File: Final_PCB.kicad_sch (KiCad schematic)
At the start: 31 parts, among them J1 USB_C_Receptacle_USB2.0_16P, J2 Conn_ARM_SWD_TagConnect_TC2030, J3 DE15_Pins_HighDensity_Mountin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, SW1 SW_Push, U1 RP2040, U2 USBLC6-2SC6, U3 SPX3819M5-L-3-3, Y1 12MHz

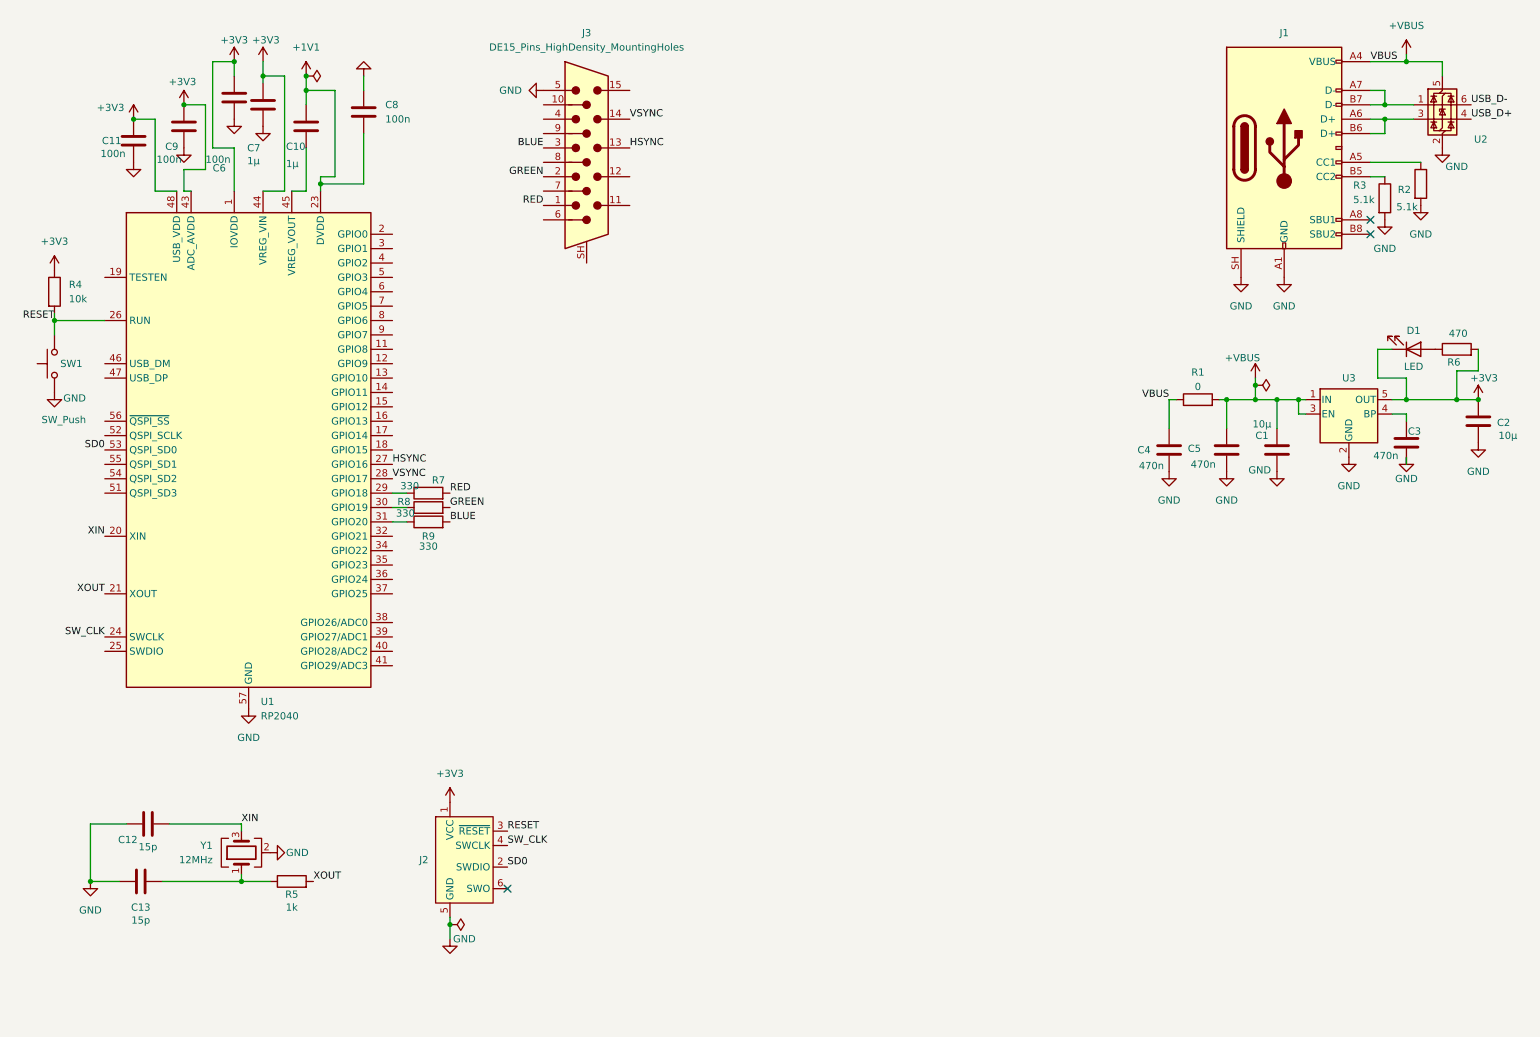
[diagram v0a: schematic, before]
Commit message: Routing almost done
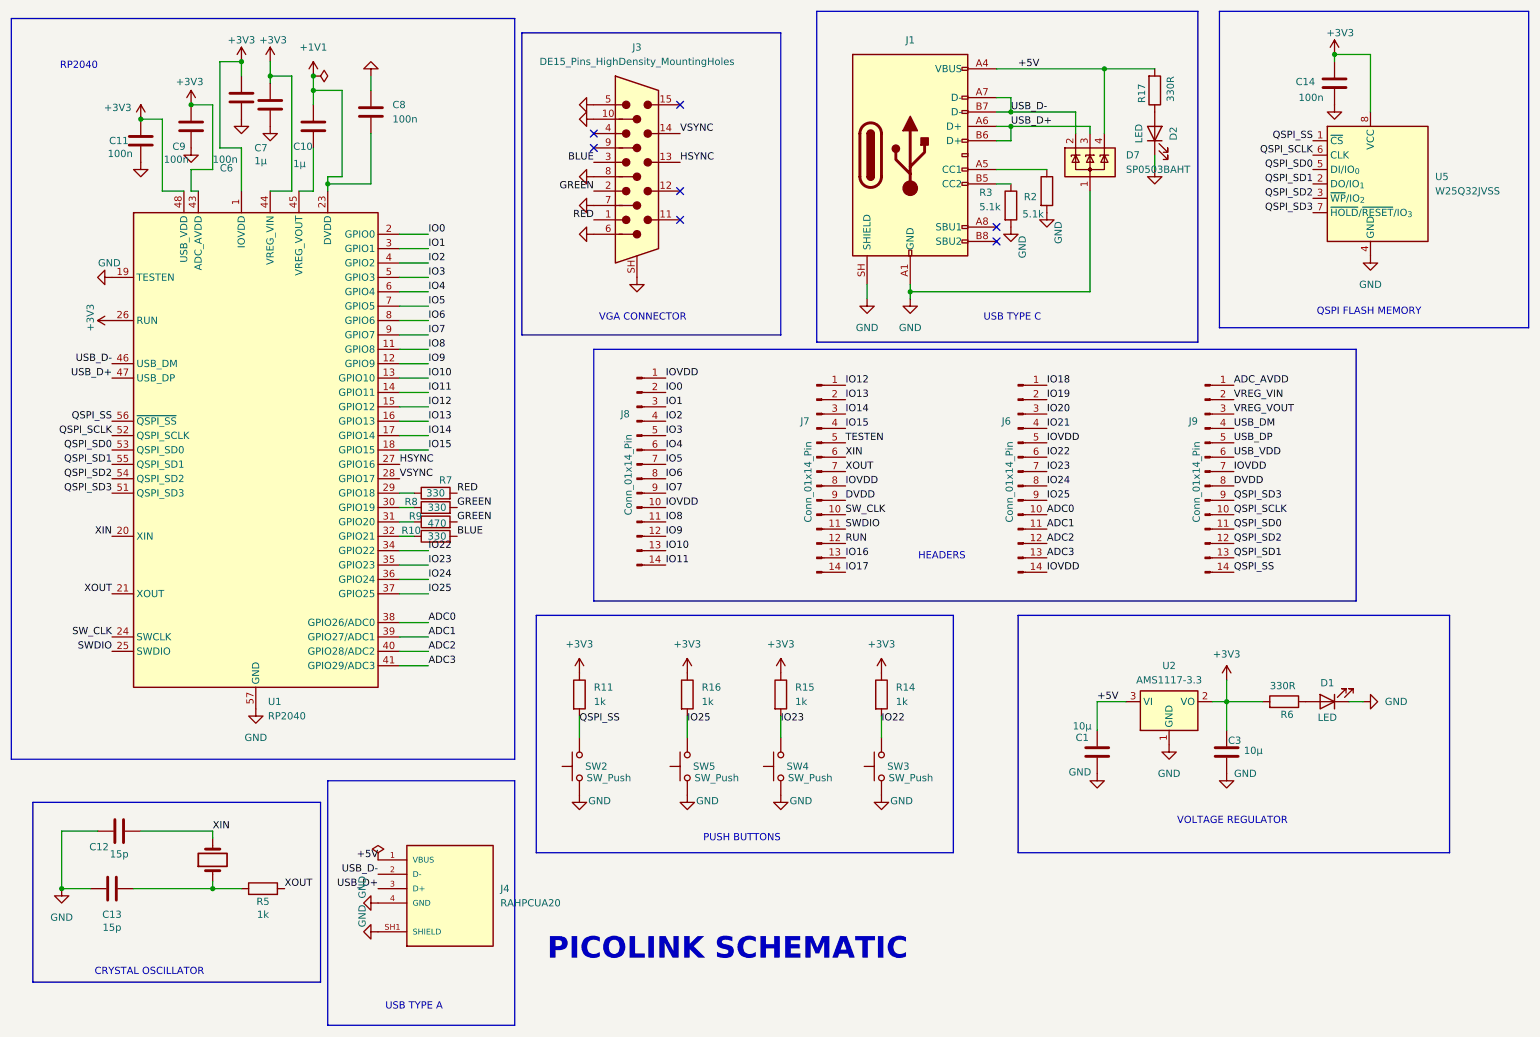
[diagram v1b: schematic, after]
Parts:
- removed C2: 10µ, Capacitor_SMD:C_0603_1608Metric, symbol Device:C
- removed C4, C5: 470n, Capacitor_SMD:C_0603_1608Metric, symbol Device:C
- removed J2: Conn_ARM_SWD_TagConnect_TC2030, Connector:Tag-Connect_TC2030-IDC-FP_2x03_P1.27mm_Vertical, symbol Connector:Conn_ARM_SWD_TagConnect_TC2030
- removed R1: 0, Resistor_SMD:R_0603_1608Metric, symbol Device:R
- removed R4: 10k, Resistor_SMD:R_0603_1608Metric, symbol Device:R
- removed SW1: SW_Push, Button_Switch_SMD:SW_SPST_B3U-1000P, symbol Switch:SW_Push
- removed U2: USBLC6-2SC6, Package_TO_SOT_SMD:SOT-23-6, symbol Power_Protection:USBLC6-2SC6
- removed U3: SPX3819M5-L-3-3, Package_TO_SOT_SMD:SOT-23-5, symbol Regulator_Linear:SPX3819M5-L-3-3
- removed Y1: 12MHz, Crystal:Crystal_SMD_5032-4Pin_5.0x3.2mm, symbol Device:Crystal_GND24
- added C14: 100n, Capacitor_SMD:C_0805_2012Metric, symbol Device:C
- added D2: LED, LED_SMD:LED_0805_2012Metric, symbol Device:LED
- added D7: SP0503BAHT, Package_TO_SOT_SMD:SOT-143, symbol Power_Protection:SP0503BAHT
- added J4: RAHPCUA20, RAHPCUA20:SWITCHCRAFT_RAHPCUA20, symbol RAHPCUA20:RAHPCUA20
- added J6, J7, J8, J9: Conn_01x14_Pin, Connector_PinHeader_1.27mm:PinHeader_1x14_P1.27mm_Vertical, symbol Connector:Conn_01x14_Pin
- added R10: 330, Resistor_SMD:R_0805_2012Metric, symbol Device:R
- added R11, R14, R15, R16: 1k, Resistor_SMD:R_0805_2012Metric, symbol Device:R
- added R17: 330R, Resistor_SMD:R_0805_2012Metric, symbol Device:R
- added SW2, SW3, SW4, SW5: SW_Push, Button_Switch_SMD:SW_SPST_B3U-1000P, symbol Switch:SW_Push
- added U2: AMS1117-3.3, Package_TO_SOT_SMD:SOT-223-3_TabPin2, symbol Regulator_Linear:AMS1117-3.3
- added U5: W25Q32JVSS, Package_SO:SOIC-8_5.3x5.3mm_P1.27mm, symbol Memory_Flash:W25Q32JVSS
- added Y2: Crystal, Crystal:Crystal_SMD_5032-2Pin_5.0x3.2mm, symbol Device:Crystal
- C1, C10, C11, C12, C13, C6, C7, C8, C9: footprint Capacitor_SMD:C_0603_1608Metric -> Capacitor_SMD:C_0805_2012Metric
- C3: value 470n -> 10µ; footprint Capacitor_SMD:C_0603_1608Metric -> Capacitor_SMD:C_0805_2012Metric
- J1: footprint Connector_USB:USB_C_Receptacle_G-Switch_GT-USB-7010ASV -> Connector_USB:USB_C_Receptacle_GCT_USB4105-xx-A_16P_TopMnt_Horizontal
- J3: footprint (none) -> Connector_Dsub:DSUB-15-HD_Socket_Horizontal_P2.29x1.90mm_EdgePinOffset3.03mm_Housed_MountingHolesOffset4.94mm
- R2, R3, R5: footprint Resistor_SMD:R_0603_1608Metric -> Resistor_SMD:R_0805_2012Metric
- R6: value 470 -> 330R; footprint Resistor_SMD:R_0603_1608Metric -> Resistor_SMD:R_0805_2012Metric
- R7, R8: footprint (none) -> Resistor_SMD:R_0805_2012Metric
- R9: value 330 -> 470; footprint (none) -> Resistor_SMD:R_0805_2012Metric
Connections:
- net RESET is gone; now on net +3V3: U1.26 (RUN)
- net +3V3: now also C3.1, C14.1, R11.1, R14.1, R15.1, R16.1, U2.2 (VO), U5.8 (VCC); no longer D1.1 (K)
- net BLUE: now also R10.2; no longer R9.2
- net GND: now also D1.1 (K), J3.10, J3.6, J3.7, J3.8, J3.SH, U1.19 (TESTEN), C14.2, D2.1 (K), D7.1 (A), J4.4 (GND), J4.SH1 (SHIELD), J4.SH2 (SHIELD), SW2.1, SW3.1, SW4.1, SW5.1, U2.1 (GND), U5.4 (GND)
- net GREEN: now also R9.2
- net SW_CLK: now also J7.10 (Pin_10)
- net USB_D+: now also J1.A6 (D+), J1.B6 (D+), U1.47 (USB_DP), D7.3 (K), J4.3 (D+)
- net USB_D-: now also J1.A7 (D-), J1.B7 (D-), U1.46 (USB_DM), D7.2 (K), J4.2 (D-)
- net XIN: now also J7.6 (Pin_6), Y2.2
- net XOUT: now also J7.7 (Pin_7)
- net at C13.2, R5.1: now also Y2.1
- net IO8: now reaches U1.11 (GPIO8)
- net IO8: now also J8.11 (Pin_11)
- net IO9: now reaches U1.12 (GPIO9)
- net IO9: now also J8.12 (Pin_12)
- net IO10: now reaches U1.13 (GPIO10)
- net IO10: now also J8.13 (Pin_13)
- net IO11: now reaches U1.14 (GPIO11)
- net IO11: now also J8.14 (Pin_14)
- net IO12: now reaches U1.15 (GPIO12)
- net IO12: now also J7.1 (Pin_1)
- net IO13: now reaches U1.16 (GPIO13)
- net IO13: now also J7.2 (Pin_2)
- net IO14: now reaches U1.17 (GPIO14)
- net IO14: now also J7.3 (Pin_3)
- net IO15: now reaches U1.18 (GPIO15)
- net IO15: now also J7.4 (Pin_4)
- net IO0: now reaches U1.2 (GPIO0)
- net IO0: now also J8.2 (Pin_2)
- net SWDIO: now reaches U1.25 (SWDIO)
- net SWDIO: now also J7.11 (Pin_11)
- net IO1: now reaches U1.3 (GPIO1)
- net IO1: now also J8.3 (Pin_3)
- net at U1.32 (GPIO21): now also R10.1
- net IO22: now reaches U1.34 (GPIO22)
- net IO22: now also J6.6 (Pin_6), R14.2, SW3.2
- net IO23: now reaches U1.35 (GPIO23)
- net IO23: now also J6.7 (Pin_7), R15.2, SW4.2
- net IO24: now reaches U1.36 (GPIO24)
- net IO24: now also J6.8 (Pin_8)
- net IO25: now reaches U1.37 (GPIO25)
- net IO25: now also J6.9 (Pin_9), R16.2, SW5.2
- net ADC0: now reaches U1.38 (GPIO26/ADC0)
- net ADC0: now also J6.10 (Pin_10)
- net ADC1: now reaches U1.39 (GPIO27/ADC1)
- net ADC1: now also J6.11 (Pin_11)
- net IO2: now reaches U1.4 (GPIO2)
- net IO2: now also J8.4 (Pin_4)
- net ADC2: now reaches U1.40 (GPIO28/ADC2)
- net ADC2: now also J6.12 (Pin_12)
- net ADC3: now reaches U1.41 (GPIO29/ADC3)
- net ADC3: now also J6.13 (Pin_13)
- net IO3: now reaches U1.5 (GPIO3)
- net IO3: now also J8.5 (Pin_5)
- net QSPI_SD3: now reaches U1.51 (QSPI_SD3)
- net QSPI_SD3: now also J9.9 (Pin_9), U5.7 (~{HOLD}/~{RESET}/IO_{3})
- net QSPI_SCLK: now reaches U1.52 (QSPI_SCLK)
- net QSPI_SCLK: now also J9.10 (Pin_10), U5.6 (CLK)
- net QSPI_SD2: now reaches U1.54 (QSPI_SD2)
- net QSPI_SD2: now also J9.12 (Pin_12), U5.3 (~{WP}/IO_{2})
- net QSPI_SD1: now reaches U1.55 (QSPI_SD1)
- net QSPI_SD1: now also J9.13 (Pin_13), U5.2 (DO/IO_{1})
- net QSPI_SS: now reaches U1.56 (~{QSPI_SS})
- net QSPI_SS: now also J9.14 (Pin_14), R11.2, SW2.2, U5.1 (~{CS})
- net IO4: now reaches U1.6 (GPIO4)
- net IO4: now also J8.6 (Pin_6)
- net IO5: now reaches U1.7 (GPIO5)
- net IO5: now also J8.7 (Pin_7)
- net IO6: now reaches U1.8 (GPIO6)
- net IO6: now also J8.8 (Pin_8)
- net IO7: now reaches U1.9 (GPIO7)
- net IO7: now also J8.9 (Pin_9)
- net +VBUS renamed +5V
- net +5V: now also D7.4 (K), J4.1 (VBUS), R17.2, U2.3 (VI)
- net SD0 renamed QSPI_SD0
- net QSPI_SD0: now also J9.11 (Pin_11), U5.5 (DI/IO_{0})
- new net: D2.2 (A), R17.1
- new net ADC_AVDD: J9.1 (Pin_1)
- new net DVDD: J7.9 (Pin_9), J9.8 (Pin_8)
- new net IO16: J7.13 (Pin_13)
- new net IO17: J7.14 (Pin_14)
- new net IO18: J6.1 (Pin_1)
- new net IO19: J6.2 (Pin_2)
- new net IO20: J6.3 (Pin_3)
- new net IO21: J6.4 (Pin_4)
- new net IOVDD: J6.14 (Pin_14), J6.5 (Pin_5), J7.8 (Pin_8), J8.1 (Pin_1), J8.10 (Pin_10), J9.7 (Pin_7)
- new net RUN: J7.12 (Pin_12)
- new net TESTEN: J7.5 (Pin_5)
- new net USB_DM: J9.4 (Pin_4)
- new net USB_DP: J9.5 (Pin_5)
- new net USB_VDD: J9.6 (Pin_6)
- new net VREG_VIN: J9.2 (Pin_2)
- new net VREG_VOUT: J9.3 (Pin_3)
- no-connect marks 3 -> 7
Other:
- note added: "CRYSTAL OSCILLATOR"
- note added: "HEADERS"
- note added: "PICOLINK SCHEMATIC"
- note added: "PUSH BUTTONS"
- note added: "QSPI FLASH MEMORY"
- note added: "RP2040"
- note added: "USB TYPE A"
- note added: "USB TYPE C"
- note added: "VGA CONNECTOR"
- note added: "VOLTAGE REGULATOR"
- title: (none) -> PicoLink
- moved on the sheet: C1, C10, C11, C12, C13, C3, C6, C7, C8, C9, D1, J1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

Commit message: Routing done and silkscreen added
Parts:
- J4: footprint RAHPCUA20:SWITCHCRAFT_RAHPCUA20 -> Connector_USB:USB_A_TE_292303-7_Horizontal
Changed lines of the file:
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@@
 			)
 		)
-		(property "Footprint" "RAHPCUA20:SWITCHCRAFT_RAHPCUA20"
+		(property "Footprint" "Connector_USB:USB_A_TE_292303-7_Horizontal"
 			(at 91.44 170.18 0)
 			(hide yes)
